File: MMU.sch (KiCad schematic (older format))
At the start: 8 parts, among them U18 74LS08, U2 74LS138, U3 MMU

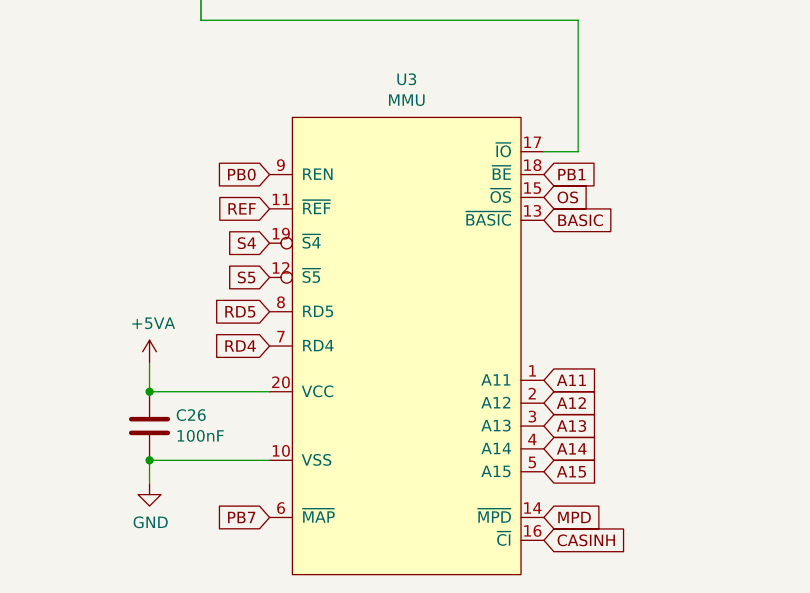
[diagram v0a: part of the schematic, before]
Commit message: SIMM update
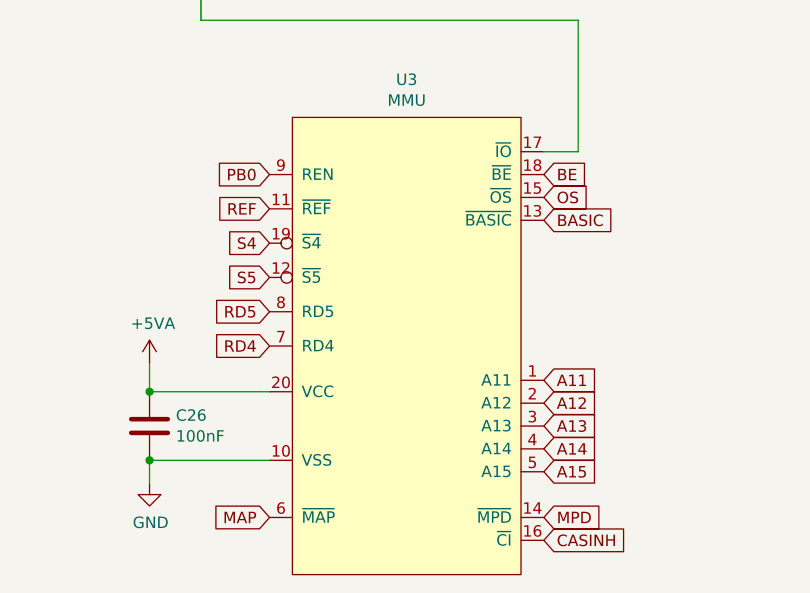
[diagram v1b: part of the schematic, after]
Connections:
- net PB1 renamed BE
- net PB7 renamed MAP
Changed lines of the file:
@@
 EESchema Schematic File Version 4
-LIBS:Atari 130XE-cache
+LIBS:Atari 130XE 1MB-cache
 EELAYER 29 0
 EELAYER END
 $Descr A4 11693 8268
 encoding utf-8
-Sheet 14 15
+Sheet 14 16
 Title ""
 Date ""
@@
 Wire Wire Line
 	1475 2175 1475 2275
-Text GLabel 4850 5750 0    50   Input ~ 0
-PB7
 Text GLabel 4850 5000 0    50   Input ~ 0
 RD4
@@
 Text GLabel 4850 4250 0    50   Input ~ 0
 PB0
-Text GLabel 6050 4250 2    50   Input ~ 0
-PB1
 Text GLabel 6050 4350 2    50   Input ~ 0
 OS
@@
 Text GLabel 5875 2750 2    50   Input ~ 0
 D7XX
+Text GLabel 6050 4250 2    50   Input ~ 0
+BE
+Text GLabel 4850 5750 0    50   Input ~ 0
+MAP
 $EndSCHEMATC
